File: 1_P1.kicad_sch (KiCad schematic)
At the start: 22 parts, among them SW1 RESET, SW2 RUN/STOP, SW3 SI, U1 74HC14, U2 IM6101, U3 2,4576 Mhz

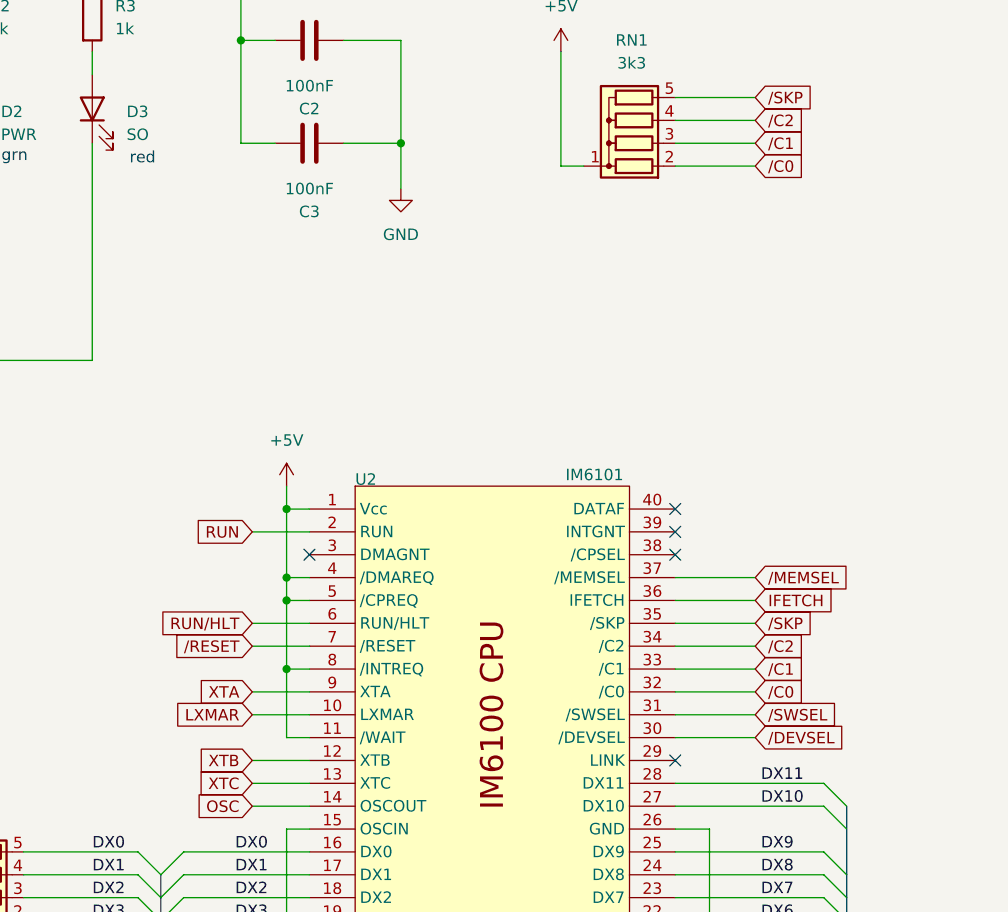
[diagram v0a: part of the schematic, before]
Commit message: HID board finalizing
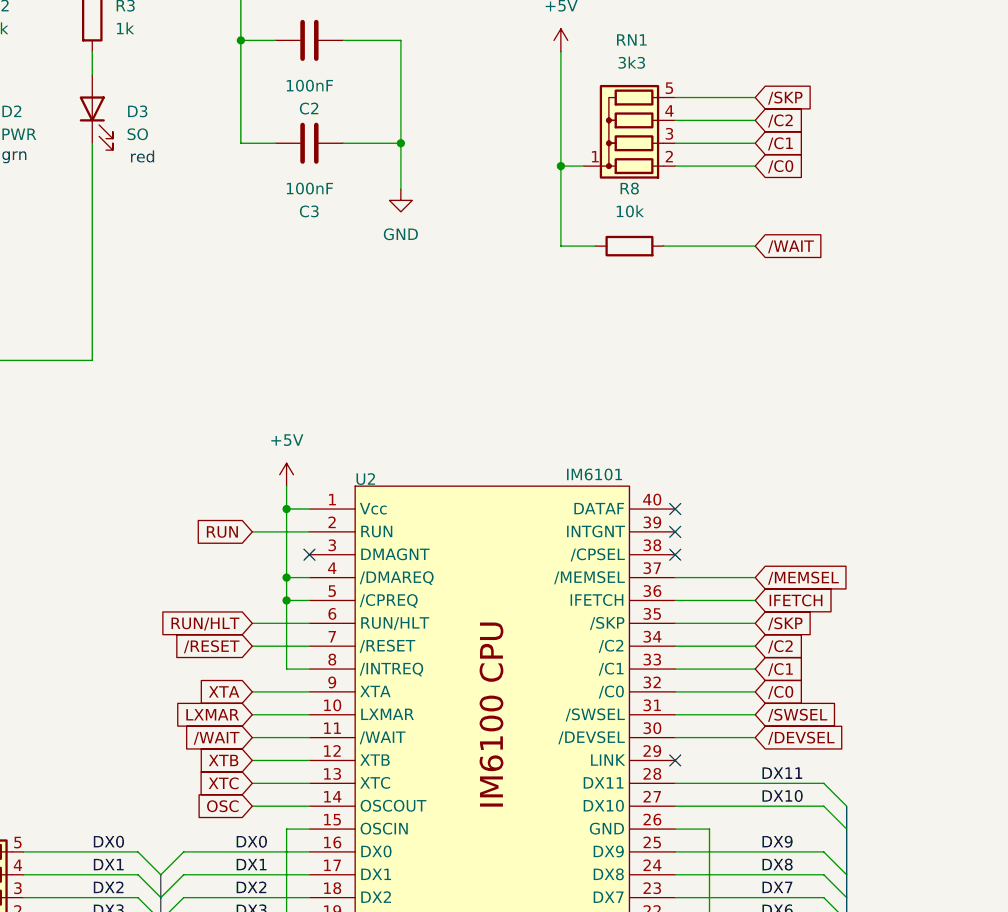
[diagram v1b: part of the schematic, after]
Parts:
- added R8: 10k, Resistor_THT:R_Axial_DIN0207_L6.3mm_D2.5mm_P7.62mm_Horizontal, symbol Device:R
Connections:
- net +5V: now also R8.1; no longer U2.11 (/WAIT)
- new net /WAIT: R8.2, U2.11 (/WAIT)
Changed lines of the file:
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@@
 	)
 	(junction
-		(at 175.26 114.3)
+		(at 187.96 55.88)
 		(diameter 0)
 		(color 0 0 0 0)
 	)
 	(junction
-		(at 187.96 55.88)
+		(at 124.46 33.02)
 		(diameter 0)
 		(color 0 0 0 0)
 	)
 	(junction
-		(at 124.46 33.02)
+		(at 205.74 58.42)
 		(diameter 0)
 		(color 0 0 0 0)
@@
 	(wire
 		(pts
+			(xy 171.45 121.92) (xy 177.8 121.92)
+		)
+		(stroke
+			(width 0)
+			(type default)
+		)
+	)
+	(wire
+		(pts
 			(xy 163.83 142.24) (xy 177.8 142.24)
 		)
@@
 	(wire
 		(pts
-			(xy 177.8 121.92) (xy 175.26 121.92)
-		)
-		(stroke
-			(width 0)
-			(type default)
-		)
-	)
-	(wire
-		(pts
 			(xy 95.25 74.93) (xy 88.9 74.93)
 		)
@@
 	(wire
 		(pts
+			(xy 205.74 67.31) (xy 209.55 67.31)
+		)
+		(stroke
+			(width 0)
+			(type default)
+		)
+	)
+	(wire
+		(pts
 			(xy 139.7 55.88) (xy 139.7 60.96)
 		)
@@
 	(wire
 		(pts
+			(xy 205.74 58.42) (xy 205.74 67.31)
+		)
+		(stroke
+			(width 0)
+			(type default)
+		)
+	)
+	(wire
+		(pts
 			(xy 57.15 134.62) (xy 57.15 147.32)
 		)
@@
 	(wire
 		(pts
+			(xy 217.17 67.31) (xy 227.33 67.31)
+		)
+		(stroke
+			(width 0)
+			(type default)
+		)
+	)
+	(wire
+		(pts
 			(xy 132.08 111.76) (xy 139.7 111.76)
 		)
@@
 	(wire
 		(pts
-			(xy 175.26 121.92) (xy 175.26 114.3)
-		)
-		(stroke
-			(width 0)
-			(type default)
-		)
-	)
-	(wire
-		(pts
 			(xy 88.9 58.42) (xy 88.9 69.85)
 		)
@@
 		)
 	)
+	(global_label "{slash}WAIT"
+		(shape input)
+		(at 171.45 121.92 180)
+		(fields_autoplaced yes)
+		(effects
+			(font
+				(size 1.27 1.27)
+			)
+			(justify right)
+		)
+		(property "Intersheetrefs" "${INTERSHEET_REFS}"
+			(at 163.0219 121.92 0)
+			(effects
+				(font
+					(size 1.27 1.27)
+				)
+				(justify right)
+				(hide yes)
+			)
+		)
+	)
 	(global_label "/C0"
 		(shape input)
@@
 		)
 	)
+	(global_label "{slash}WAIT"
+		(shape input)
+		(at 227.33 67.31 0)
+		(fields_autoplaced yes)
+		(effects
+			(font
+				(size 1.27 1.27)
+			)
+			(justify left)
+		)
+		(property "Intersheetrefs" "${INTERSHEET_REFS}"
+			(at 235.7581 67.31 0)
+			(effects
+				(font
+					(size 1.27 1.27)
+				)
+				(justify left)
+				(hide yes)
+			)
+		)
+	)
 	(global_label "OSC"
 		(shape input)
@@
 					(unit 1)
 				)
+			)
+		)
+	)
+	(symbol
+		(lib_id "Device:R")
+		(at 213.36 67.31 90)
+		(unit 1)
+		(exclude_from_sim no)
+		(in_bom yes)
+		(on_board yes)
+		(dnp no)
+		(fields_autoplaced yes)
+		(property "Reference" "R8"
+			(at 213.36 60.96 90)
+			(effects
+				(font
+					(size 1.27 1.27)
+				)
+			)
+		)
+		(property "Value" "10k"
+			(at 213.36 63.5 90)
+			(effects
+				(font
+					(size 1.27 1.27)
+				)
+			)
+		)
+		(property "Footprint" "Resistor_THT:R_Axial_DIN0207_L6.3mm_D2.5mm_P7.62mm_Horizontal"
+			(at 213.36 69.088 90)
+			(effects
+				(font
+					(size 1.27 1.27)
+				)
+				(hide yes)
+			)
+		)
+		(property "Datasheet" "~"
+			(at 213.36 67.31 0)
+			(effects
+				(font
+					(size 1.27 1.27)
+				)
+				(hide yes)
+			)
+		)
+		(property "Description" "Resistor"
+			(at 213.36 67.31 0)
+			(effects
+				(font
+					(size 1.27 1.27)
+				)
+				(hide yes)
+			)
+		)
+		(pin "1"
+		)
+		(pin "2"
+		)
+		(instances
+			(project "IM6100 SAMPLER_v3"
+				(path "/2a7e57b3-5bbf-459b-bd73-b2368ad605c6/95e48f54-28ef-4b60-833e-b06f16a55f82"
+					(reference "R8")
+					(unit 1)
+				)
